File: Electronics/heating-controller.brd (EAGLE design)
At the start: 53 x 55.9 mm, 19 parts, among them IC1 AP1117T33L-U, Q1 IRLB8721PBF

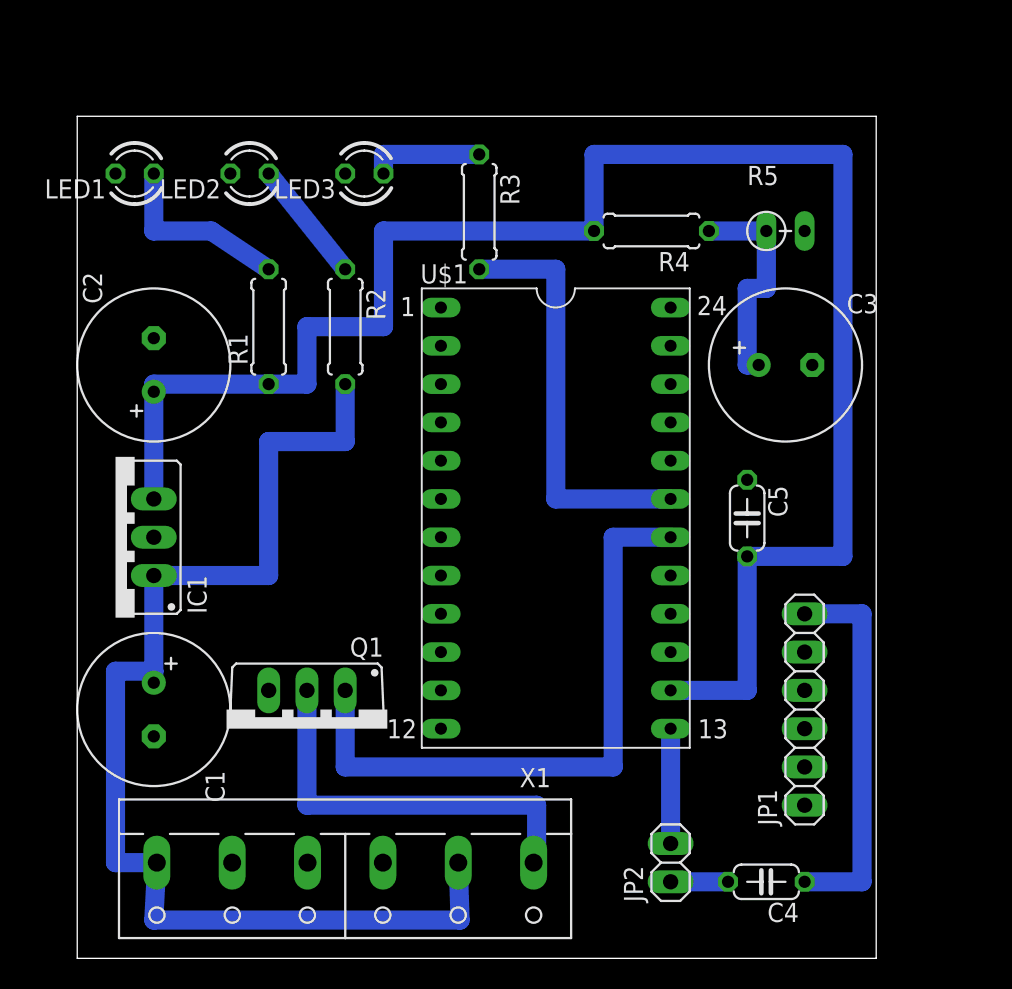
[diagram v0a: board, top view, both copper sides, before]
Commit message: First version of PCB complete.
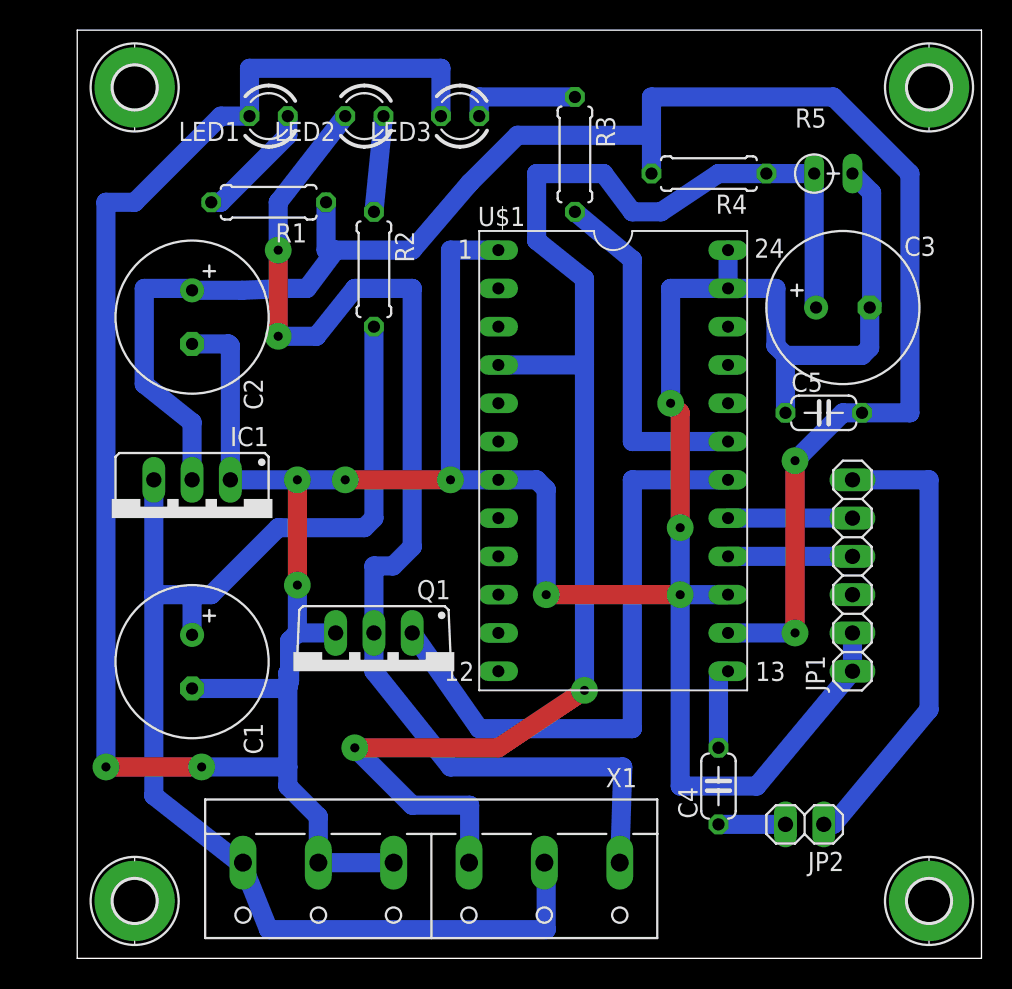
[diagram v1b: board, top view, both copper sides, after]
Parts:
- added H1, H2, H3, H4: MOUNT-PAD-ROUND2.8, holes:2,8-PAD
- IC1: value AP1117T33L-U -> AP1117 (3v3); device v-reg:78XXS -> v-reg:79XXS
- moved LED1 9.67 mm to (12.7, 55.9)
- moved JP1 9.44 mm to (51.4, 25.4)
- moved JP2 9.25 mm to (48.3, 8.89), turned to 180 degrees
- moved C5 8.64 mm to (49.5, 36.2), turned to 0 degrees
- moved LED2 8.52 mm to (19.1, 55.9)
- moved R1 8.26 mm to (12.7, 50.2), turned to 180 degrees
- moved R3 7.41 mm to (33.0, 53.3)
- moved LED3 7.41 mm to (25.4, 55.9)
- moved C4 7.10 mm to (42.5, 11.4), turned to 90 degrees
- moved Q1 5.85 mm to (19.7, 19.1)
- moved X1 5.71 mm to (23.5, 5.08)
- moved U$1 5.39 mm to (35.6, 33.0)
- moved C3 5.39 mm to (50.8, 43.2)
- moved R4 5.39 mm to (41.9, 52.1)
- moved IC1 5.24 mm to (7.62, 29.2), turned to 180 degrees
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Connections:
- removed net N$13: C4.2, JP2.1
- new net N$8: C4.1, JP2.2
- net +12V: now also IC1.OUT; no longer IC1.IN
- net N$12: now also JP2.1; no longer C4.1
- net N$14: now also C4.2; no longer JP2.2
- net VCC: now also IC1.IN; no longer IC1.OUT
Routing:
- net GND: track 0.00 -> 279.0 mm, vias 0 -> 10
- net N$1: track 14.7 -> 100.4 mm, vias 0 -> 2
- net N$3: track 26.9 -> 79.7 mm, vias 0 -> 2
- net +12V: track 78.4 -> 88.5 mm
- net N$9: track 0.00 -> 8.26 mm
- net N$10: track 0.00 -> 8.26 mm
- net VCC: track 115.6 -> 121.4 mm, vias 0 -> 2
- net N$12: track 25.4 -> 30.9 mm
- net N$2: track 27.9 -> 23.4 mm
- net N$8: track 0.00 -> 4.45 mm
- net N$4: track 12.2 -> 8.19 mm
- net N$13: track 3.81 -> 0.00 mm
- net N$14: track 7.62 -> 5.71 mm
- net N$5: track 8.13 -> 6.38 mm
- net N$7: track 41.9 -> 40.8 mm
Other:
- board size 53 x 55.9 mm -> 60 x 61.6 mm
